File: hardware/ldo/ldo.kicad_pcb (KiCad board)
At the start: 2 copper layers, 20 parts, among them U1 AMS1117-3.3

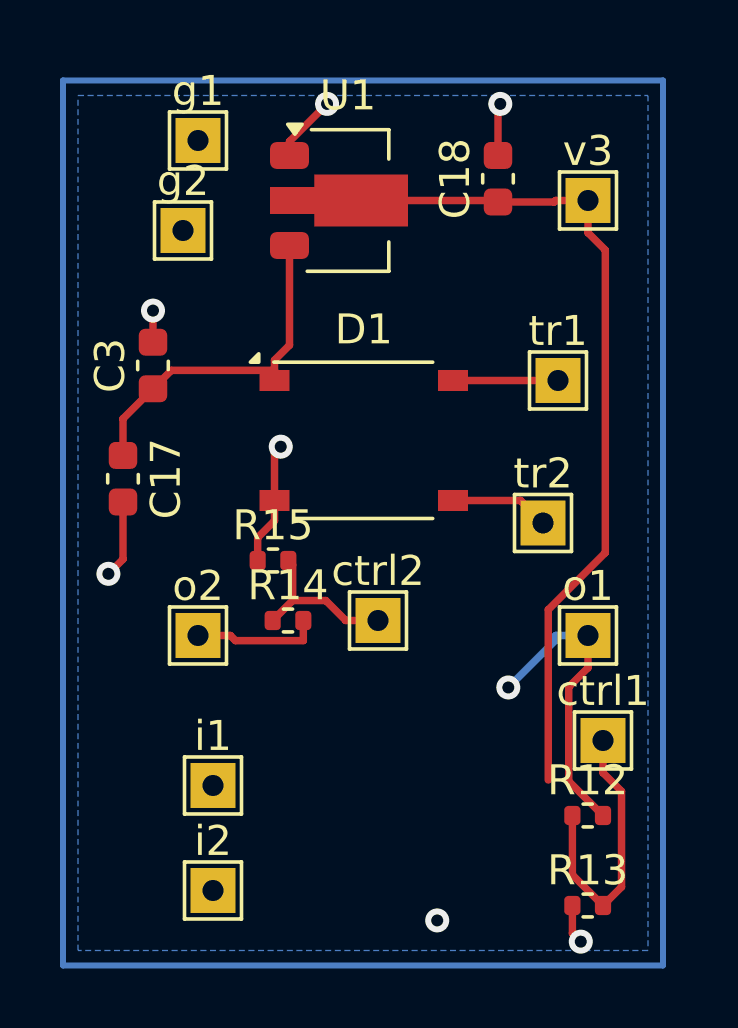
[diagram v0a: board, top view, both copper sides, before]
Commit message: wip
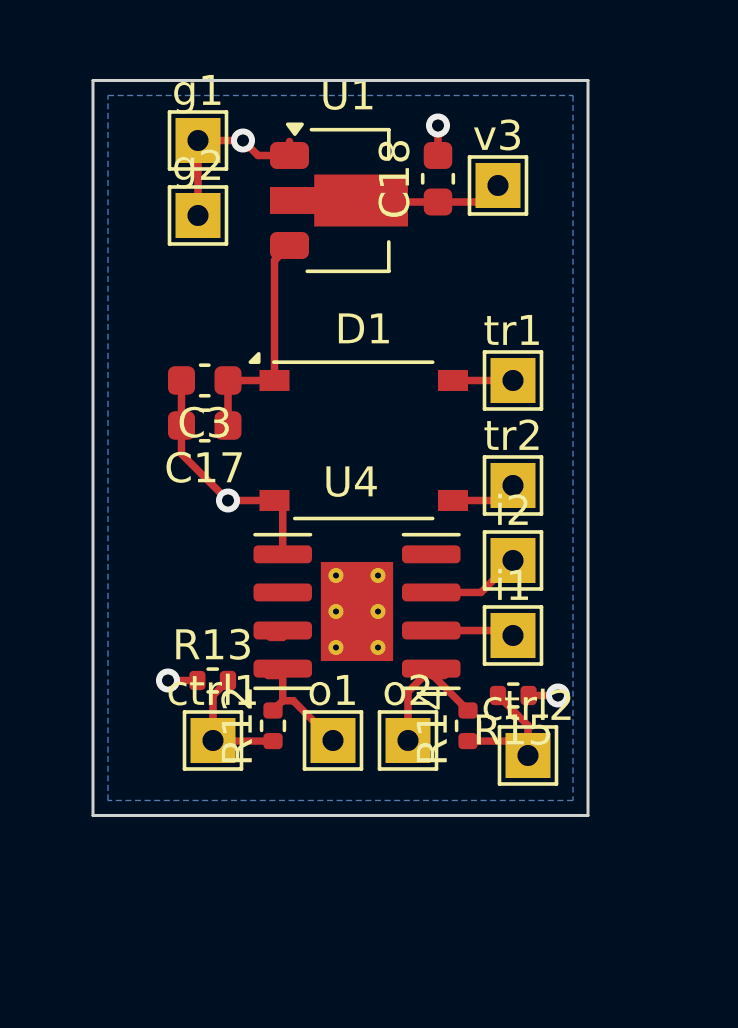
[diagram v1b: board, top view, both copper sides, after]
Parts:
- added U4: BDR6133, Library:SOIC-8-1EP_3.9x4.9mm_P1.27mm_EP2.41x3.3mm_ThermalVias, F.Cu at (110.3, 55.2)
- moved i2 14.9 mm to (115.5, 53.5)
- moved R13 14.6 mm to (105.5, 57.5)
- moved ctrl1 13.0 mm to (105.5, 59.5)
- moved i1 11.2 mm to (115.5, 56.0)
- moved R12 10.9 mm to (107.5, 59.0), turned to 90 degrees
- moved o1 9.19 mm to (109.5, 59.5)
- moved R15 9.19 mm to (115.5, 58.0), turned to 180 degrees
- moved o2 7.83 mm to (112.0, 59.5)
- moved R14 6.95 mm to (114.0, 59.0), turned to 90 degrees
- moved ctrl2 6.73 mm to (116.0, 60.0)
- moved C17 3.25 mm to (105.2, 49.0), turned to 180 degrees
- moved v3 3.04 mm to (115.0, 41.0)
- moved C18 2.00 mm to (113.0, 40.8)
- moved C3 1.80 mm to (105.2, 47.5), turned to 180 degrees
- moved tr2 1.60 mm to (115.5, 51.0)
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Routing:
- net VCC: track 30.2 -> 7.11 mm
- net Net-(U4-OUTA): track 10.2 -> 4.25 mm, vias 1 -> 0
- net Net-(R12-Pad1): track 9.43 -> 4.92 mm
- net GND: track 13.7 -> 18.0 mm, vias 7 -> 5
- net Net-(D1-+): track 11.7 -> 8.40 mm
- net Net-(U4-INB): track 0.00 -> 3.17 mm
- net Net-(U4-INA): track 0.00 -> 2.79 mm
- net Net-(D1-Pad4): track 3.50 -> 2.00 mm
- net Net-(D1-Pad3): track 3.31 -> 2.21 mm
- net Net-(R14-Pad1): track 5.46 -> 4.61 mm
- net Net-(U4-OUTB): track 4.25 -> 5.06 mm
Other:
- board outline added: 16.5 x 24.5 mm
